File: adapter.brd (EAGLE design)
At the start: 47.9 x 48.2 mm, 28 parts, among them Q1 BS170, Q2 BS170, Q3 BS170, Q4 BS170, X2 KUSBVX

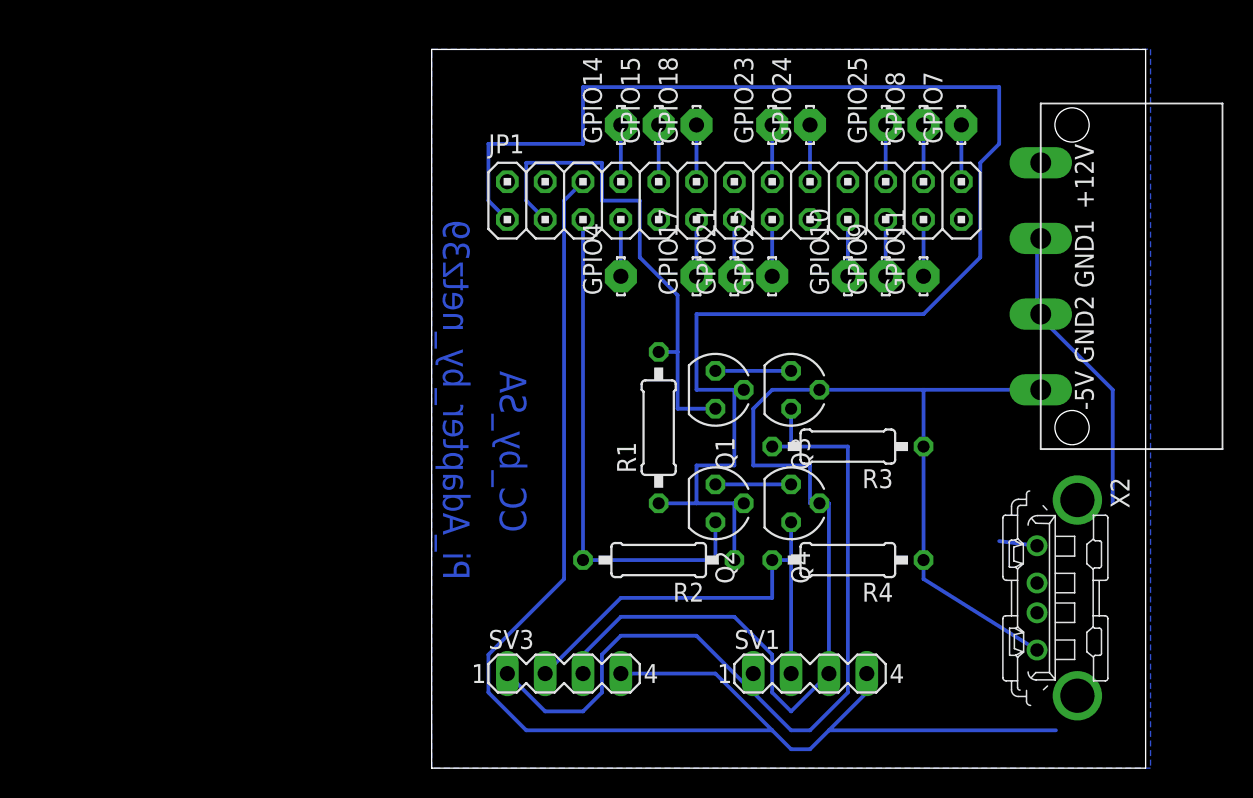
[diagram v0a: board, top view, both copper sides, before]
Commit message: letzte Anpassungen zum Ätzen
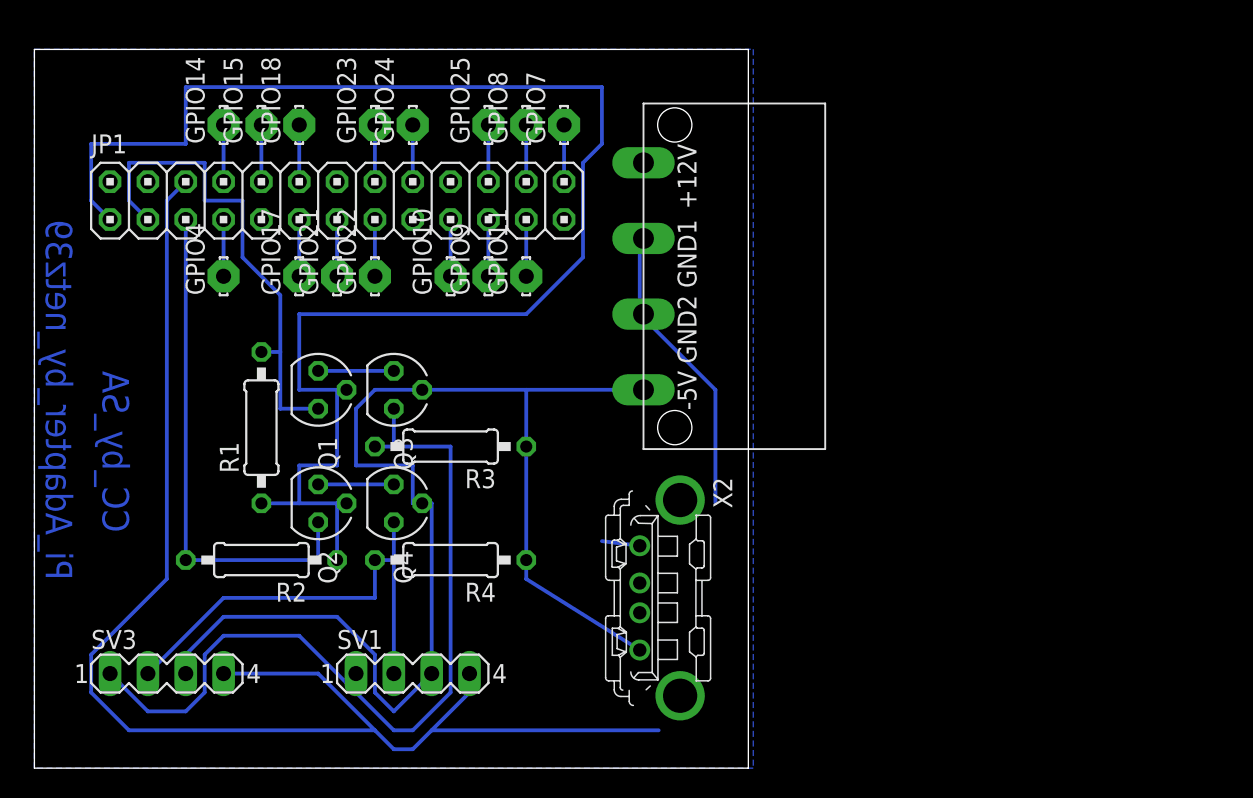
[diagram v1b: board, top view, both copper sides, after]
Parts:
- moved GPIO14 26.7 mm to (22.9, 43.2)
- moved GPIO15 26.7 mm to (25.4, 43.2)
- moved GPIO25 26.7 mm to (40.6, 43.2)
- moved GPIO4 26.7 mm to (22.9, 33.0)
- moved GPIO7 26.7 mm to (45.7, 43.2)
- moved GPIO9 26.7 mm to (40.6, 33.0)
- moved Q1 26.7 mm to (29.2, 25.4)
- moved Q2 26.7 mm to (29.2, 17.8)
- moved Q3 26.7 mm to (34.3, 25.4)
- moved Q4 26.7 mm to (34.3, 17.8)
- moved R1 26.7 mm to (25.4, 22.9)
- moved R2 26.7 mm to (25.4, 14.0)
- moved X2 26.7 mm to (50.8, 11.4)
- moved GPIO17 26.7 mm to (27.9, 33.0)
- moved GPIO18 26.7 mm to (27.9, 43.2)
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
